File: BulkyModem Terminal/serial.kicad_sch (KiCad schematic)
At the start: 12 parts, among them J2 RS-232, J5 TTL, U2 74HCT244, U3 MAX232

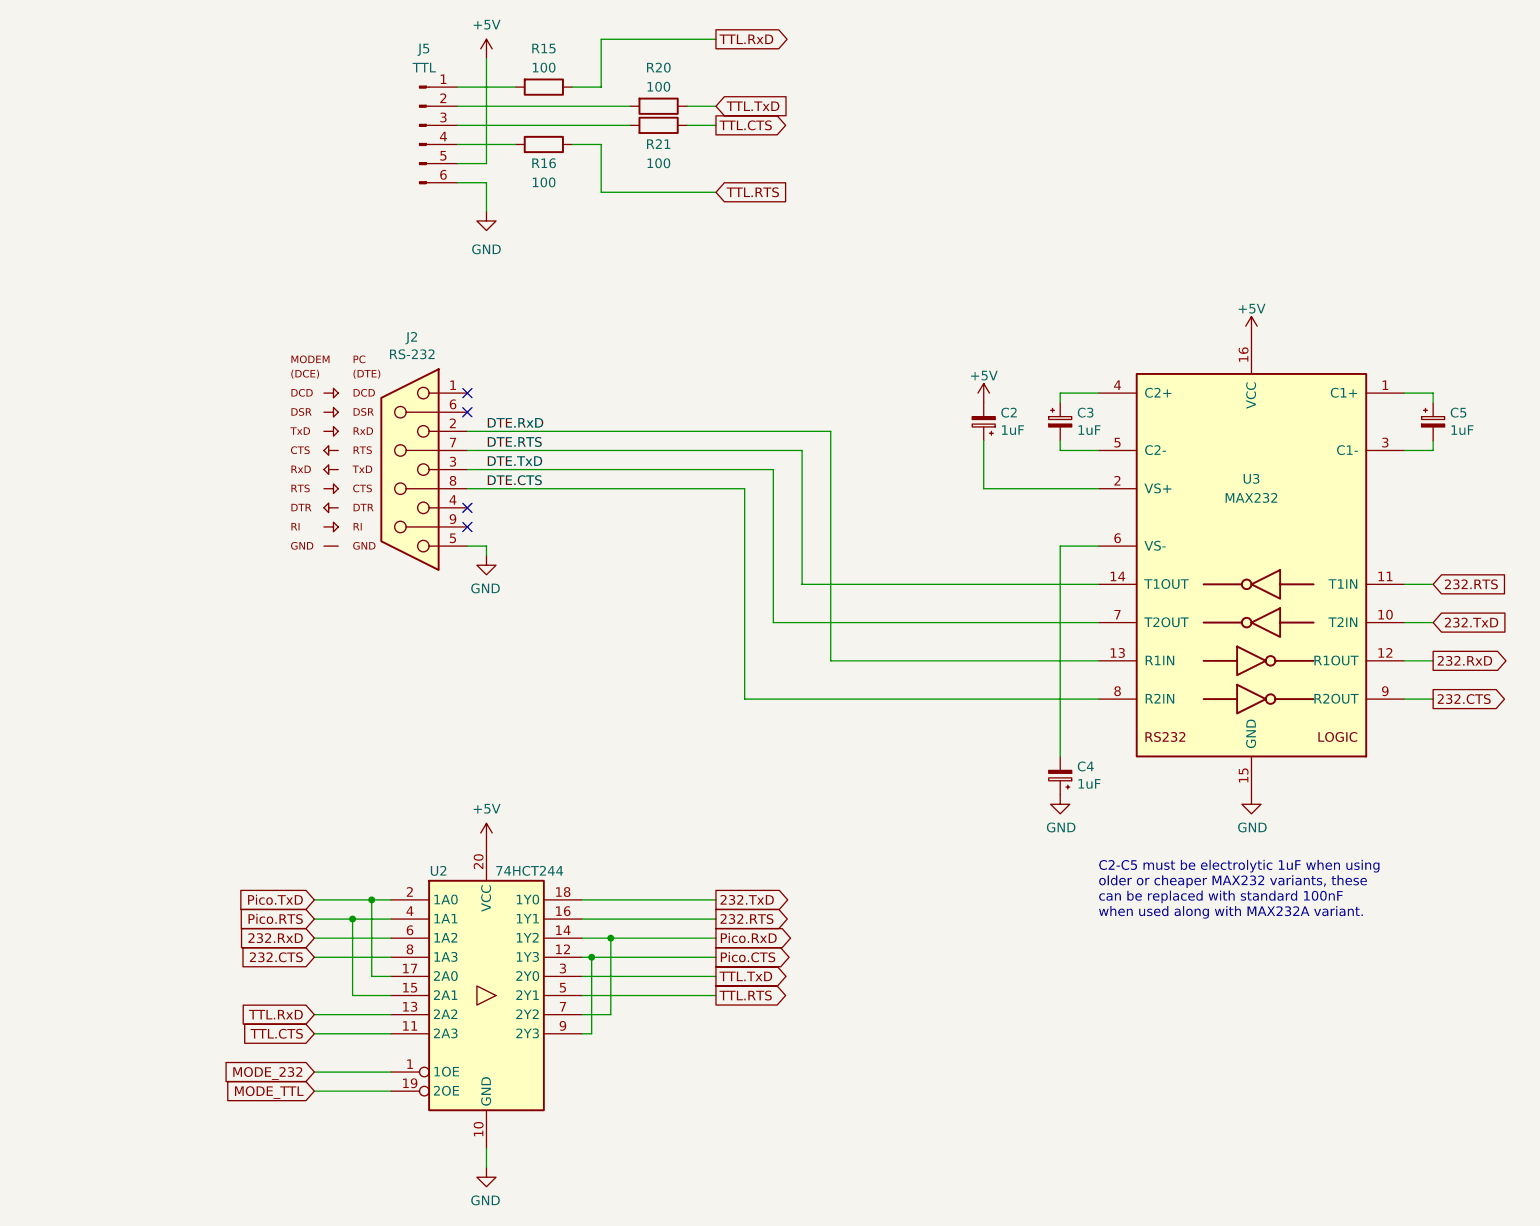
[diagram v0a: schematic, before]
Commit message: Part of a layout
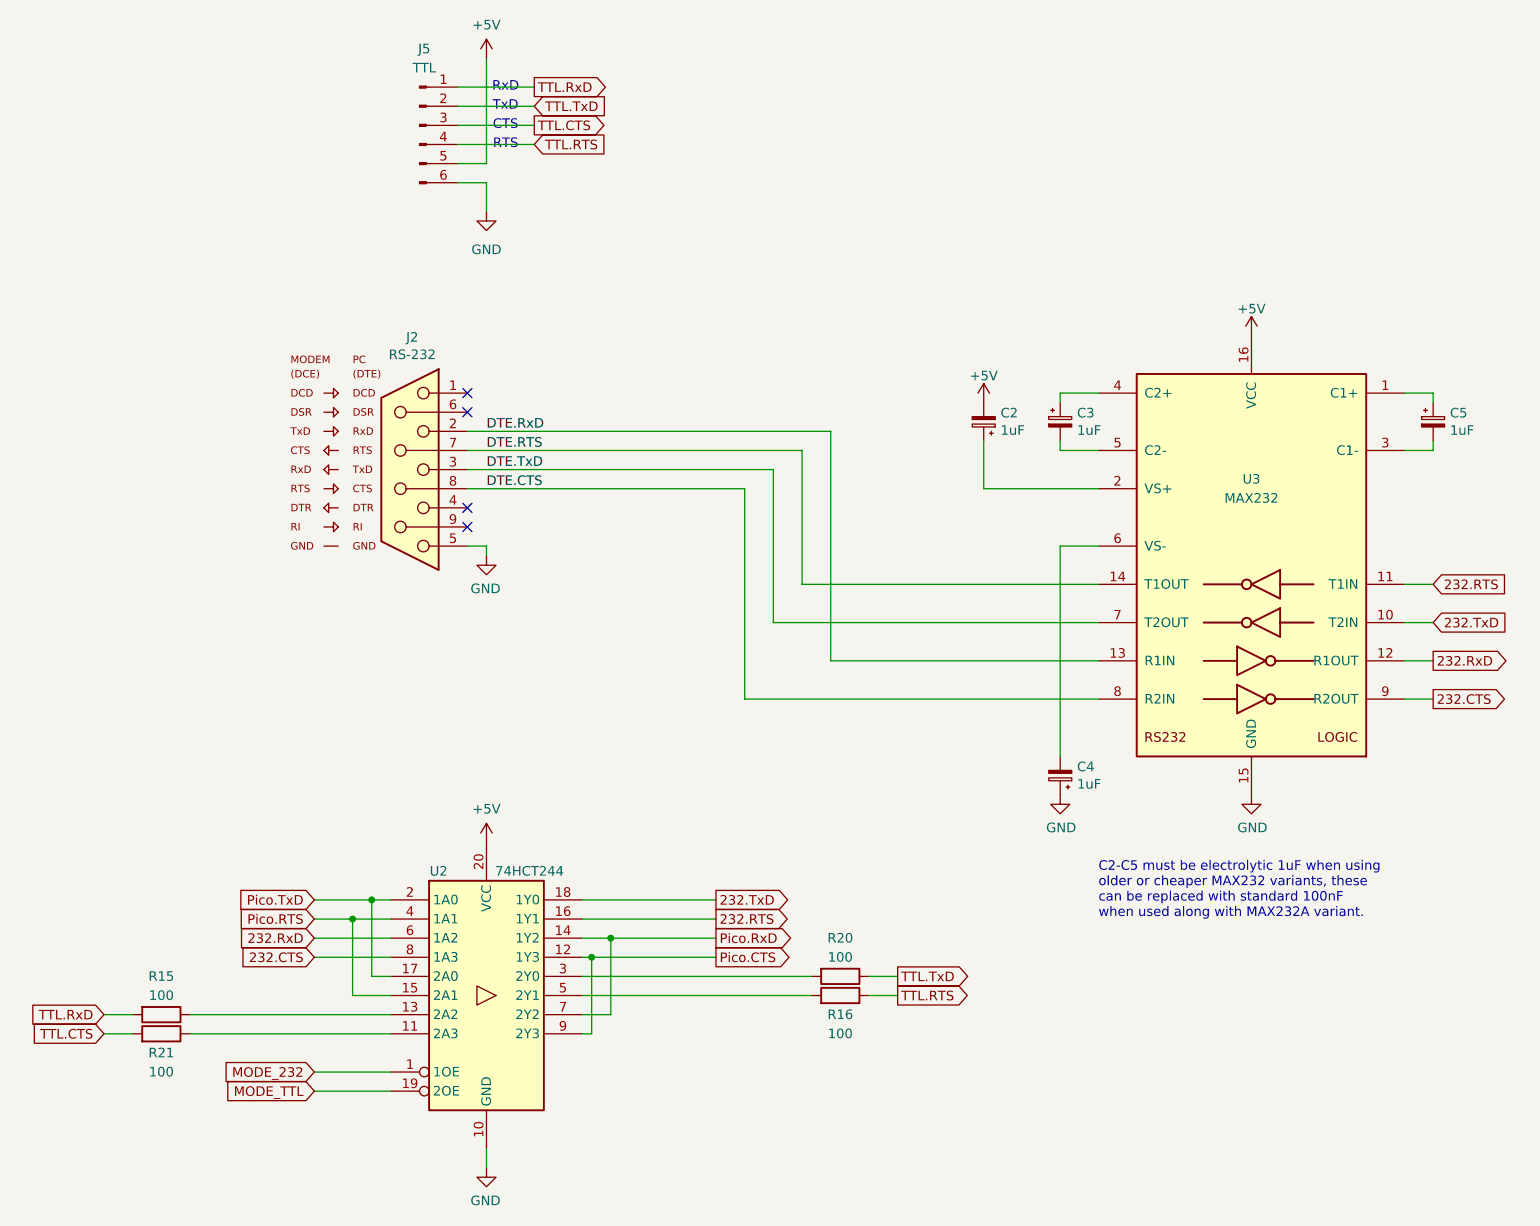
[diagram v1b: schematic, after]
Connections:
- net TTL.CTS: now also J5.3 (Pin_3), R21.2; no longer R21.1, U2.11 (2A3)
- net TTL.RTS: now also J5.4 (Pin_4); no longer U2.5 (2Y1)
- net TTL.RxD: now also J5.1 (Pin_1), R15.2; no longer R15.1, U2.13 (2A2)
- net TTL.TxD: now also J5.2 (Pin_2); no longer U2.3 (2Y0)
- net at R16.2: now also U2.5 (2Y1); no longer J5.4 (Pin_4)
- net at R20.2: now also U2.3 (2Y0); no longer J5.2 (Pin_2)
- new net: R15.1, U2.13 (2A2)
- new net: R21.1, U2.11 (2A3)
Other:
- note added: "CTS"
- note added: "RTS"
- note added: "RxD"
- note added: "TxD"
- moved on the sheet: R15
